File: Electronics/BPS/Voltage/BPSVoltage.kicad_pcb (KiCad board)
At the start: 2 copper layers, 58.4 x 59.7 mm, 72 parts, among them J1 Conn1, J2 Conn2, J3 Conn_01x06, J4 Conn_01x07, Q1 BSS308PE, Q10 BSS308PE, Q11 BSS308PE, Q12 BSS308PE, Q13 BSS308PE, Q2 BSS308PE, Q3 BSS308PE, Q4 BSS308PE, Q5 NSV1C201MZ4, Q6 BSS308PE, Q7 BSS308PE, Q8 BSS308PE, Q9 BSS308PE, U1 LTC6811-1, U2 HX1188FNL

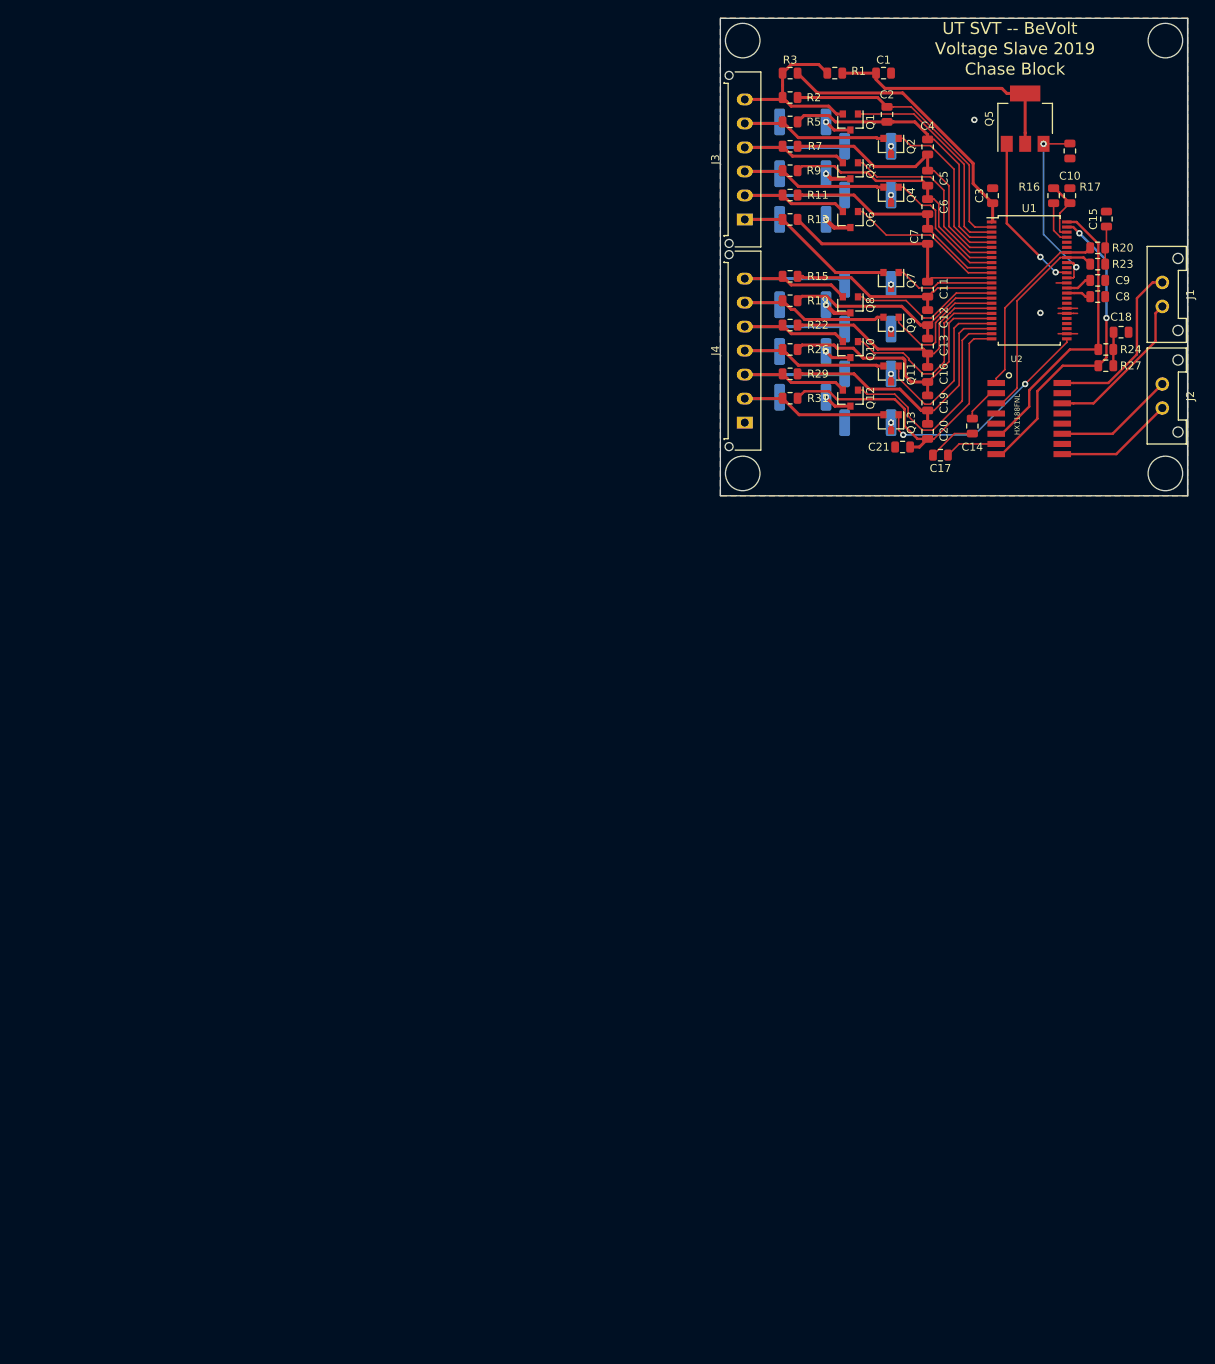
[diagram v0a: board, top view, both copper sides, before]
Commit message: Finished up revision 2 of the board.
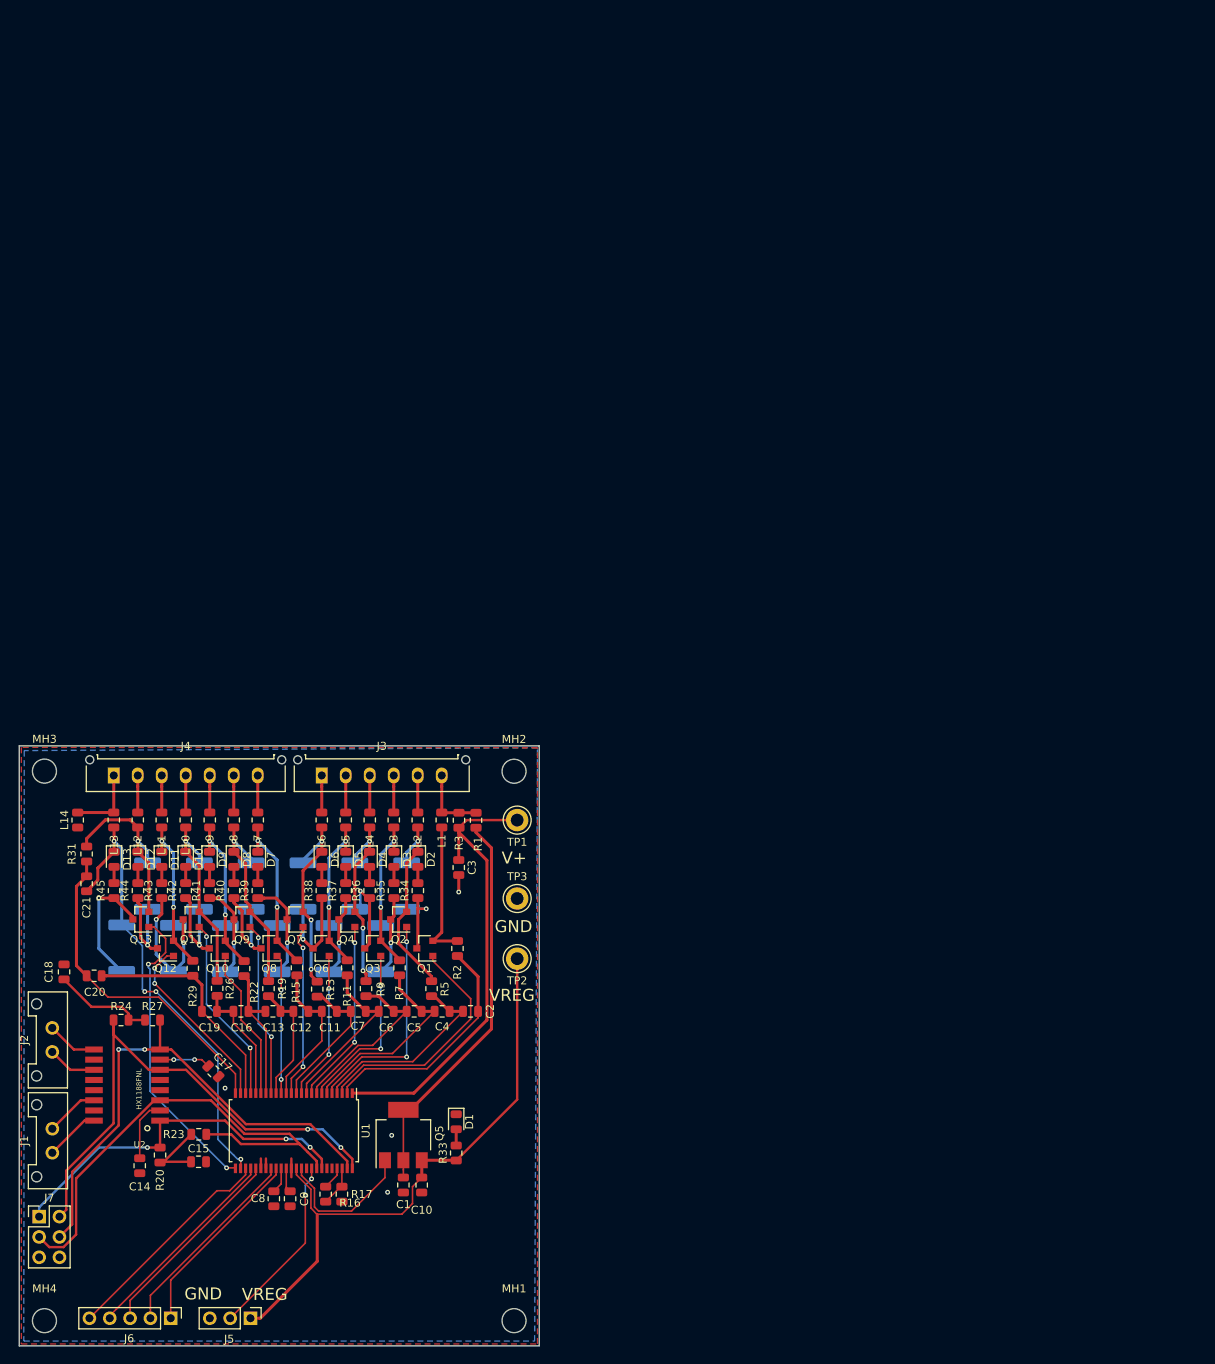
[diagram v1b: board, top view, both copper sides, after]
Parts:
- added D1: LED, LED_SMD:LED_0805_2012Metric, F.Cu at (134.6, 157.0)
- added D10: LED, LED_SMD:LED_0805_2012Metric, F.Cu at (100.8, 124.2)
- added D11: LED, LED_SMD:LED_0805_2012Metric, F.Cu at (97.8, 124.2)
- added D12: LED, LED_SMD:LED_0805_2012Metric, F.Cu at (94.8, 124.2)
- added D13: LED, LED_SMD:LED_0805_2012Metric, F.Cu at (91.9, 124.2)
- added D2: LED, LED_SMD:LED_0805_2012Metric, F.Cu at (129.8, 124.2)
- added D3: LED, LED_SMD:LED_0805_2012Metric, F.Cu at (126.8, 124.2)
- added D4: LED, LED_SMD:LED_0805_2012Metric, F.Cu at (123.8, 124.2)
- added D5: LED, LED_SMD:LED_0805_2012Metric, F.Cu at (120.8, 124.2)
- added D6: LED, LED_SMD:LED_0805_2012Metric, F.Cu at (117.8, 124.2)
- added D7: LED, LED_SMD:LED_0805_2012Metric, F.Cu at (109.8, 124.2)
- added D8: LED, LED_SMD:LED_0805_2012Metric, F.Cu at (106.8, 124.2)
- added D9: LED, LED_SMD:LED_0805_2012Metric, F.Cu at (103.8, 124.2)
- added J5: Conn_01x03, Connector_PinHeader_2.54mm:PinHeader_1x03_P2.54mm_Vertical, F.Cu at (108.9, 181.5)
- added J6: Conn_01x05, Connector_PinHeader_2.54mm:PinHeader_1x05_P2.54mm_Vertical, F.Cu at (98.9, 181.5)
- added J7: Conn_02x03_Counter_Clockwise, Connector_PinHeader_2.54mm:PinHeader_2x03_P2.54mm_Vertical, F.Cu at (82.5, 168.8)
- added L1: Ferrite_Bead, Inductor_SMD:L_0805_2012Metric, F.Cu at (132.8, 119.3)
- added L10: Ferrite_Bead, Inductor_SMD:L_0805_2012Metric, F.Cu at (100.8, 119.3)
- added L11: Ferrite_Bead, Inductor_SMD:L_0805_2012Metric, F.Cu at (97.8, 119.3)
- added L12: Ferrite_Bead, Inductor_SMD:L_0805_2012Metric, F.Cu at (94.8, 119.3)
- added L13: Ferrite_Bead, Inductor_SMD:L_0805_2012Metric, F.Cu at (91.8, 119.3)
- added L14: Ferrite_Bead, Inductor_SMD:L_0805_2012Metric, F.Cu at (87.3, 119.3)
- added L2: Ferrite_Bead, Inductor_SMD:L_0805_2012Metric, F.Cu at (129.8, 119.3)
- added L3: Ferrite_Bead, Inductor_SMD:L_0805_2012Metric, F.Cu at (126.8, 119.3)
- added L4: Ferrite_Bead, Inductor_SMD:L_0805_2012Metric, F.Cu at (123.8, 119.3)
- added L5: Ferrite_Bead, Inductor_SMD:L_0805_2012Metric, F.Cu at (120.8, 119.3)
- added L6: Ferrite_Bead, Inductor_SMD:L_0805_2012Metric, F.Cu at (117.8, 119.3)
- added L7: Ferrite_Bead, Inductor_SMD:L_0805_2012Metric, F.Cu at (109.8, 119.3)
- added L8: Ferrite_Bead, Inductor_SMD:L_0805_2012Metric, F.Cu at (106.8, 119.3)
- added L9: Ferrite_Bead, Inductor_SMD:L_0805_2012Metric, F.Cu at (103.8, 119.3)
- added MH1: MountingHole, MountingHole:MountingHole_3mm, F.Cu at (141.8, 181.8)
- added MH2: MountingHole, MountingHole:MountingHole_3mm, F.Cu at (141.8, 113.2)
- added MH3: MountingHole, MountingHole:MountingHole_3mm, F.Cu at (83.2, 113.2)
- added MH4: MountingHole, MountingHole:MountingHole_3mm, F.Cu at (83.2, 181.8)
- added R33: 1.5k, Resistor_SMD:R_0805_2012Metric, F.Cu at (134.6, 160.9)
- added R34: 1.2k, Resistor_SMD:R_0805_2012Metric, F.Cu at (129.8, 128.1)
- added R35: 1.2k, Resistor_SMD:R_0805_2012Metric, F.Cu at (126.8, 128.1)
- added R36: 1.2k, Resistor_SMD:R_0805_2012Metric, F.Cu at (123.8, 128.1)
- added R37: 1.2k, Resistor_SMD:R_0805_2012Metric, F.Cu at (120.8, 128.1)
- added R38: 1.2k, Resistor_SMD:R_0805_2012Metric, F.Cu at (117.8, 128.1)
- added R39: 1.2k, Resistor_SMD:R_0805_2012Metric, F.Cu at (109.8, 128.1)
- added R40: 1.2k, Resistor_SMD:R_0805_2012Metric, F.Cu at (106.8, 128.1)
- added R41: 1.2k, Resistor_SMD:R_0805_2012Metric, F.Cu at (103.8, 128.1)
- added R42: 1.2k, Resistor_SMD:R_0805_2012Metric, F.Cu at (100.8, 128.1)
- added R43: 1.2k, Resistor_SMD:R_0805_2012Metric, F.Cu at (97.8, 128.1)
- added R44: 1.2k, Resistor_SMD:R_0805_2012Metric, F.Cu at (94.8, 128.1)
- added R45: 1.2k, Resistor_SMD:R_0805_2012Metric, F.Cu at (91.9, 128.1)
- added TP1: V+, TestPoint:TestPoint_Keystone_5005-5009_Compact, F.Cu at (142.2, 119.3)
- added TP2: VREG, TestPoint:TestPoint_Keystone_5005-5009_Compact, F.Cu at (142.2, 136.6)
- added TP3: GND, TestPoint:TestPoint_Keystone_5005-5009_Compact, F.Cu at (142.2, 129.1)
- R16: value 1k -> 806
- R17: value 1k -> 1.21k
- moved J1 176.3 mm to (84.1, 160.9), turned to 90 degrees
- moved C15 163.6 mm to (102.4, 162.0), turned to 0 degrees
- moved R20 163.1 mm to (97.6, 161.1), turned to 270 degrees
- moved J2 161.9 mm to (84.1, 148.3), turned to 90 degrees
- moved R23 156.4 mm to (102.4, 158.6), turned to 180 degrees
- moved R16 154.5 mm to (118.3, 166.0), turned to 90 degrees
- moved R17 154.5 mm to (120.3, 166.0), turned to 90 degrees
- moved C18 154.4 mm to (85.6, 138.3), turned to 90 degrees
- moved C9 152.9 mm to (113.9, 166.6), turned to 270 degrees
- moved C8 152.7 mm to (111.8, 166.6), turned to 270 degrees
- moved C10 152.6 mm to (130.3, 164.9)
- moved C1 151.4 mm to (128.0, 164.9), turned to 270 degrees
- moved Q5 148.9 mm to (128.0, 158.6)
- moved R24 148.9 mm to (92.7, 144.3)
- moved R27 144.5 mm to (96.7, 144.3), turned to 180 degrees
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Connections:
- net Net-(Q1-Pad3) renamed /L11
- net Net-(Q10-Pad3) renamed /L3
- net Net-(Q11-Pad3) renamed /L2
- net Net-(Q12-Pad3) renamed /L1
- net Net-(Q13-Pad3) renamed /L0
- net Net-(Q2-Pad3) renamed /L10
- net Net-(Q3-Pad3) renamed /L9
- net Net-(Q4-Pad3) renamed /L8
- net Net-(Q6-Pad3) renamed /L7
- net Net-(Q7-Pad3) renamed /L6
- net Net-(Q8-Pad3) renamed /L5
- net Net-(Q9-Pad3) renamed /L4
- C21 pad 1: GND -> /Batt0
- J3 pad 1: /Batt7 -> Net-(J3-Pad1)
- J3 pad 2: /Batt8 -> Net-(J3-Pad2)
- J3 pad 3: /Batt9 -> Net-(J3-Pad3)
- J3 pad 4: /Batt10 -> Net-(J3-Pad4)
- J3 pad 5: /Batt11 -> Net-(J3-Pad5)
- J3 pad 6: /Batt12 -> /V12
- J4 pad 1: GND -> Net-(J4-Pad1)
- J4 pad 2: /Batt1 -> Net-(J4-Pad2)
- J4 pad 3: /Batt2 -> Net-(J4-Pad3)
- J4 pad 4: /Batt3 -> Net-(J4-Pad4)
- J4 pad 5: /Batt4 -> Net-(J4-Pad5)
- J4 pad 6: /Batt5 -> Net-(J4-Pad6)
- J4 pad 7: /Batt6 -> Net-(J4-Pad7)
- R1 pad 2: /Batt12 -> /V12
- R3 pad 1: /Batt12 -> /V12
- R32 pad 1: GND -> /Batt0
- U1 pad 26: GND -> /Batt0
- U1 pad 27: (no net) -> /GPIO1
- U1 pad 28: (no net) -> /GPIO2
- U1 pad 29: (no net) -> /GPIO3
- U1 pad 32: (no net) -> /GPIO4
- U1 pad 33: (no net) -> /GPIO5
- U1 pad 40: /VREG -> /ISOMD
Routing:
- net /Batt0: track 0.00 -> 57.9 mm, vias 0 -> 4
- net /VREG: track 25.4 -> 75.1 mm, vias 2 -> 0
- net /IMA: track 26.0 -> 63.2 mm
- net /IPB: track 36.6 -> 66.7 mm, vias 0 -> 2
- net /GPIO1: track 0.00 -> 27.8 mm
- net /GPIO2: track 0.00 -> 26.0 mm
- net /IMB: track 39.6 -> 65.4 mm
- net /GPIO3: track 0.00 -> 25.2 mm
- net /GPIO4: track 0.00 -> 25.0 mm
- net /GPIO5: track 0.00 -> 24.2 mm
- net /ISOMD: track 0.00 -> 23.0 mm, vias 0 -> 2
- net Net-(C3-Pad1): track 35.0 -> 57.8 mm
- net /IPA: track 23.6 -> 46.1 mm, vias 0 -> 3
- net Net-(C16-Pad1): track 35.3 -> 15.4 mm
- net Net-(C1-Pad1): track 30.7 -> 49.6 mm
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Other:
- board size 58.4 x 59.7 mm -> 65 x 75 mm
- board text added: "GND"
- board text added: "V+"
- board text added: "VREG"
- board text removed: "Chase Block"
- board text removed: "UT SVT -- BeVolt"
- board text removed: "Voltage Slave 2019"
